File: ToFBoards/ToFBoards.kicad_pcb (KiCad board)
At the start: 2 copper layers, 1 part, among them U1 VL53L1X

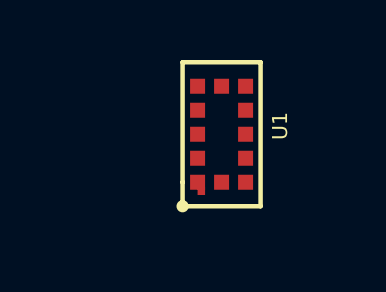
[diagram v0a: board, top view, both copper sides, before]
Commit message: ToF boards
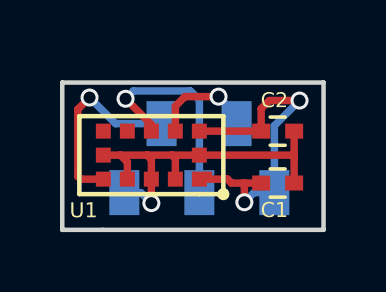
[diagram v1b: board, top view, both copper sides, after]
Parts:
- added C1: 100n, Capacitors_SMD:C_0402, F.Cu at (151.2, 105.0)
- added C2: 4.7u, Capacitors_SMD:C_0402, F.Cu at (151.2, 103.3)
- added J1: Bottom, ToFTop, B.Cu at (148.6, 103.3)
- added J2: Top, ToFBottom, B.Cu at (148.6, 105.1)
- moved U1 0.12 mm to (148.6, 104.9), turned to 90 degrees
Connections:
- U1 pad 1: Net-(U1-Pad1) -> VCC
- U1 pad 10: (no net) -> SCL
- U1 pad 11: (no net) -> VCC
- U1 pad 12: (no net) -> GND
- U1 pad 2: (no net) -> GND
- U1 pad 3: (no net) -> GND
- U1 pad 4: (no net) -> GND
- U1 pad 5: (no net) -> SIGNAL
- U1 pad 6: (no net) -> GND
- U1 pad 9: (no net) -> SDA
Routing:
- net GND: track 0.00 -> 12.6 mm, vias 0 -> 1
- net VCC: track 0.00 -> 12.1 mm, vias 0 -> 2
- net SDA: track 0.00 -> 7.22 mm, vias 0 -> 1
- net SIGNAL: track 0.00 -> 6.44 mm, vias 0 -> 1
- net SCL: track 0.00 -> 3.55 mm, vias 0 -> 1
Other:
- board outline added: 8.7 x 4.9 mm
